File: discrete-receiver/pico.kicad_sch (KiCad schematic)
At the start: 38 parts, among them SW1 Reset, U6 RP2350A, U7 W25Q128JVS, U8 NCP1117-3.3_SOT223, Y1 ABM8-272-T3

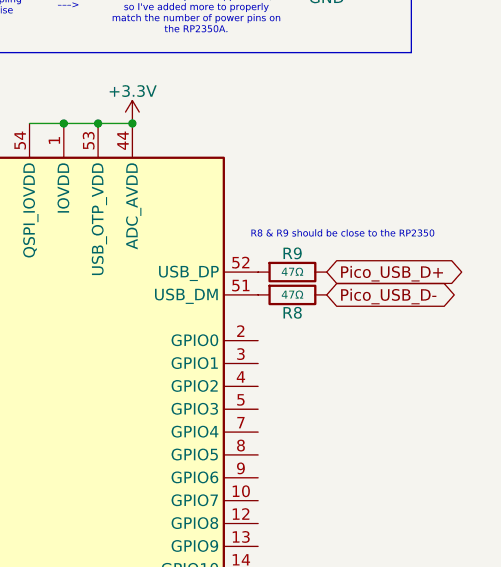
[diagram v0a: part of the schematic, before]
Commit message: update schematic for peter
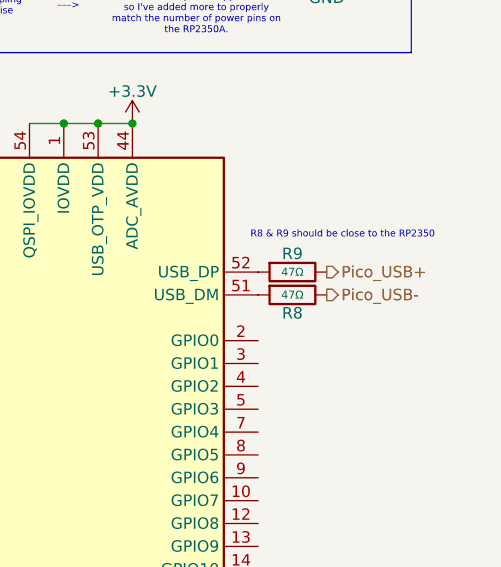
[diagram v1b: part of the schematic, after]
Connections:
- net Pico_USB_D+ renamed Pico_USB+
- net Pico_USB_D- renamed Pico_USB-
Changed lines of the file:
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@@
-		)
-	)
-	(global_label "Pico_USB_D+"
-		(shape bidirectional)
-		(at 270.51 67.31 0)
-		(fields_autoplaced yes)
-		(effects
-			(font
-				(size 1.27 1.27)
-				(thickness 0.1588)
-			)
-			(justify left)
-		)
-		(property "Intersheetrefs" "${INTERSHEET_REFS}"
-			(at 287.3065 67.31 0)
-			(hide yes)
-			(show_name no)
-			(do_not_autoplace no)
-			(effects
-				(font
-					(size 1.27 1.27)
-				)
-				(justify left)
-			)
 		)
 	)
@@
 		)
 	)
-	(global_label "Pico_USB_D-"
-		(shape bidirectional)
-		(at 270.51 69.85 0)
-		(fields_autoplaced yes)
-		(effects
-			(font
-				(size 1.27 1.27)
-				(thickness 0.1588)
-			)
-			(justify left)
-		)
-		(property "Intersheetrefs" "${INTERSHEET_REFS}"
-			(at 287.3065 69.85 0)
-			(hide yes)
-			(show_name no)
-			(do_not_autoplace no)
-			(effects
-				(font
-					(size 1.27 1.27)
-				)
-				(justify left)
-			)
-		)
-	)
 	(global_label "XIN"
 		(shape passive)
@@
 		)
 	)
+	(hierarchical_label "Pico_USB+"
+		(shape output)
+		(at 270.51 67.31 0)
+		(effects
+			(font
+				(size 1.27 1.27)
+			)
+			(justify left)
+		)
+	)
+	(hierarchical_label "Pico_USB-"
+		(shape output)
+		(at 270.51 69.85 0)
+		(effects
+			(font
+				(size 1.27 1.27)
+			)
+			(justify left)
+		)
+	)
